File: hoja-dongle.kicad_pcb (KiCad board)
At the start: 2 copper layers, 30 x 44 mm, 64 parts, among them J2 USB4080-03-A_REVA1, J3 Conn_01x04_Pin, P1 RPI-RM2, Q1 BSS138DW, Q2 BSS138DW, SW1 1TS026A-1000-0550, SW2 SW_Push, SW3 SW_Push, U1 USBLC6-2P6, U2 USBLC6-2P6, U3 USBLC6-2P6, U4 TPS630001RCR, U5 RP2350_60QFN, Y1 ABM8-272-T3

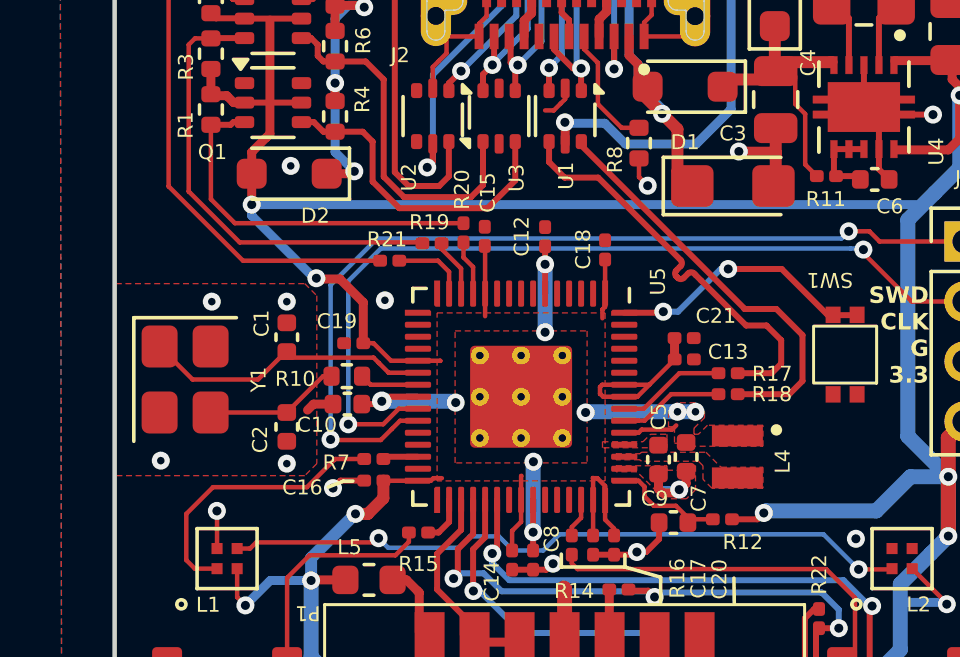
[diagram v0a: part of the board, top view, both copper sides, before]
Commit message: prod
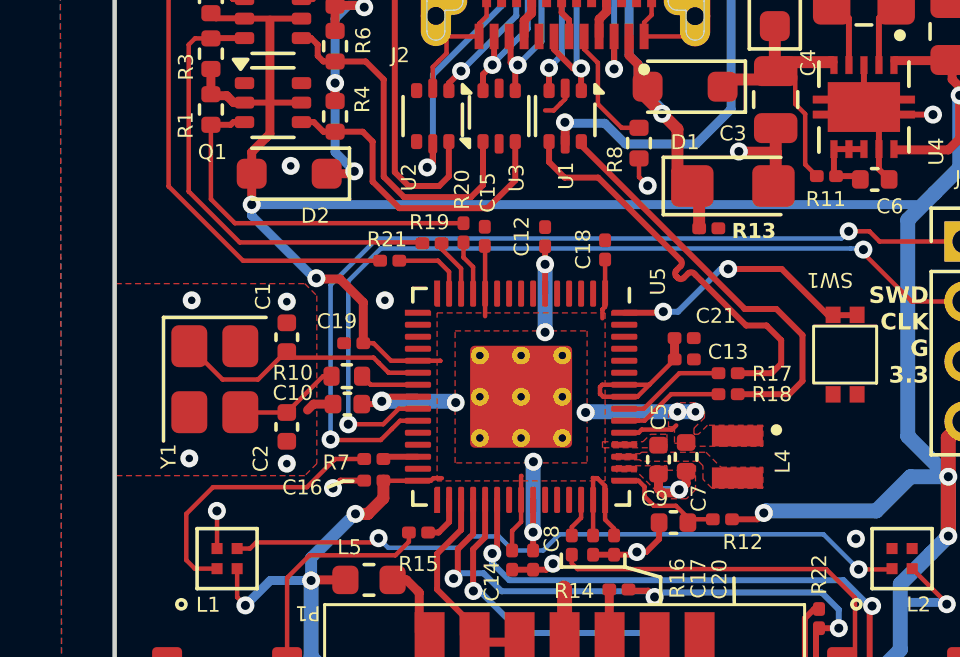
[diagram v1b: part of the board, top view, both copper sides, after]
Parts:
- added R13: 51K, Resistor_SMD:R_0201_0603Metric, F.Cu at (119.7, 39.7)
- R19, R20, R21: value 100R -> 27R
- moved Y1 0.99 mm to (103.2, 44.8)
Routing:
- net +3V3_PRE: track 31.2 -> 32.7 mm
- net XTAL_IN: track 9.67 -> 8.67 mm
- net Net-(C2-Pad1): track 4.53 -> 3.55 mm
